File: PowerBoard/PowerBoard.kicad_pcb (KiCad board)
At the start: 2 copper layers, 45 x 100 mm, 13 parts, among them U1 RDE20110S12

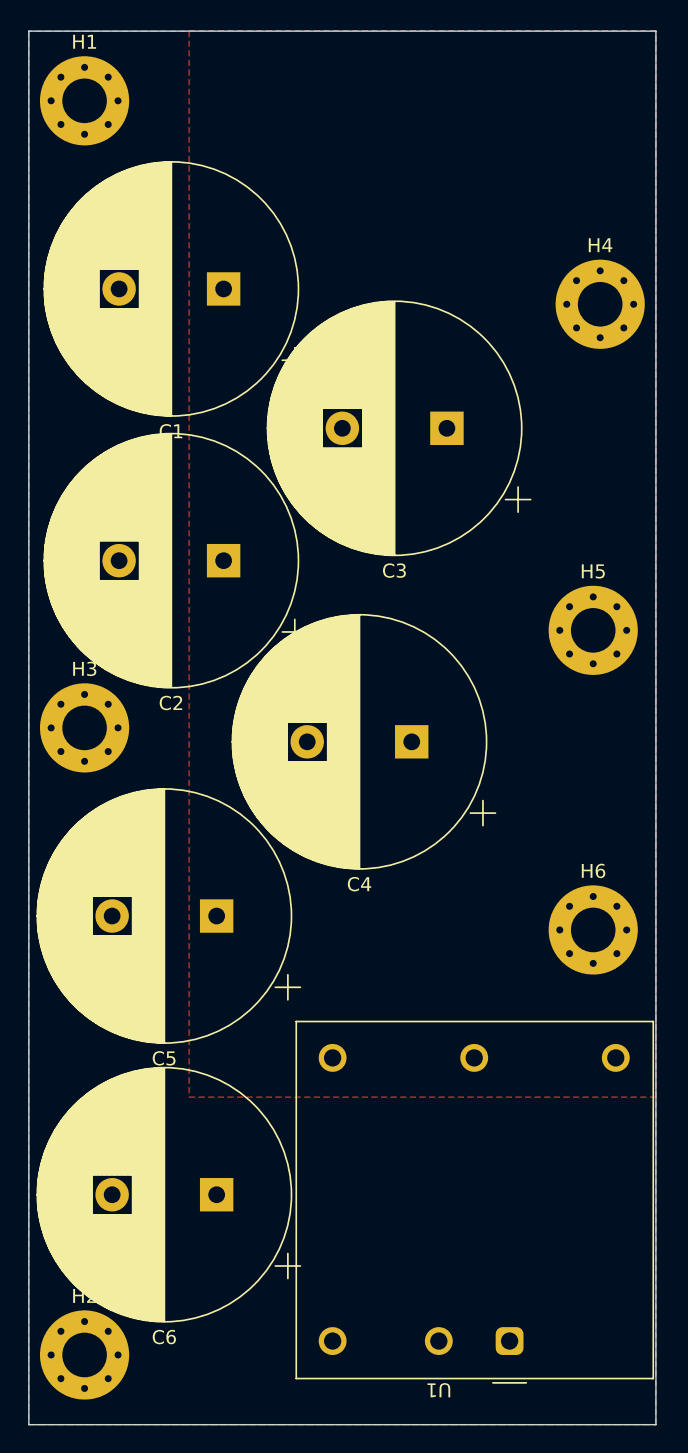
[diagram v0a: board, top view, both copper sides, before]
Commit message: cheap_board
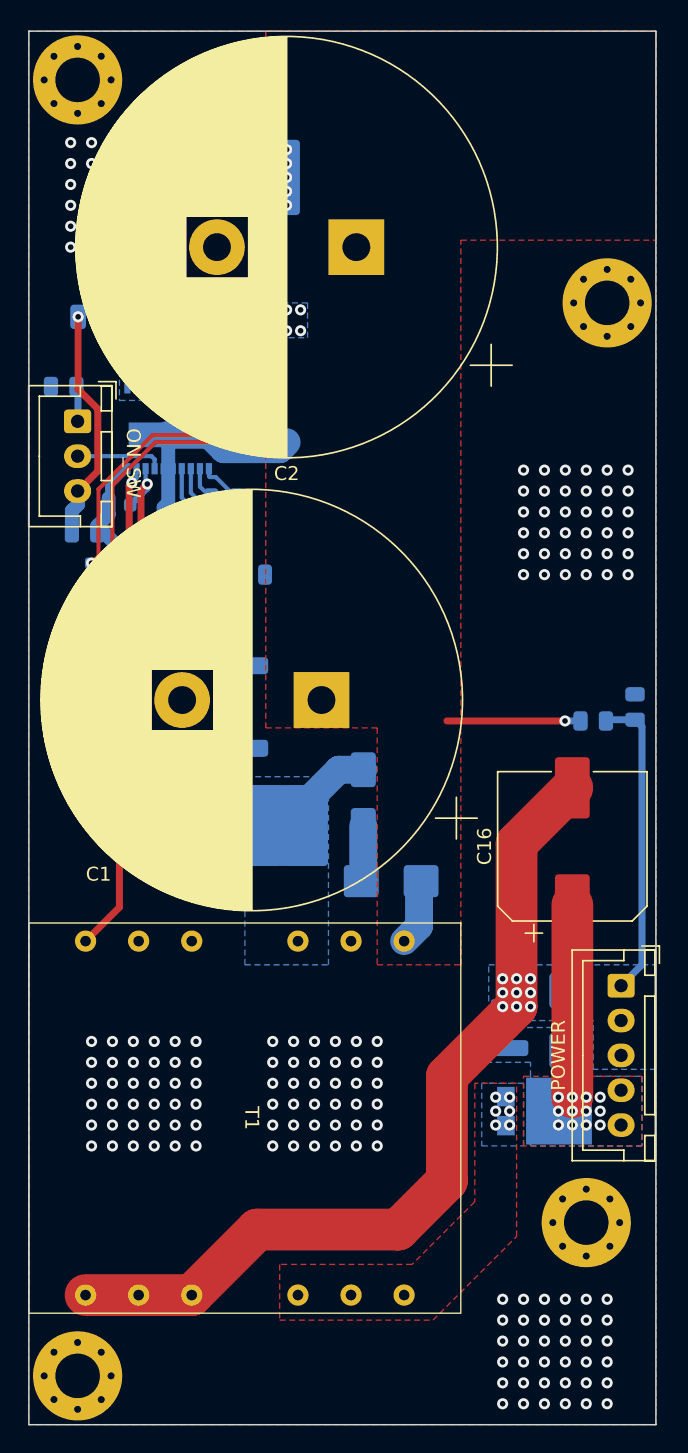
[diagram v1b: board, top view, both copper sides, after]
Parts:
- removed C3, C4, C5, C6: 680uF 200V, Capacitor_THT:CP_Radial_D18.0mm_P7.50mm
- removed H5, H6: BATT+Hole, MountingHole:MountingHole_3.2mm_M3_Pad_Via
- removed U1: RDE20110S12, Converter_DCDC:Converter_DCDC_TRACO_THN30-xxxx_THT
- added C10: 47p 25V, Capacitor_SMD:C_0805_2012Metric, B.Cu at (60.5, 87.0)
- added C11: 4.7u 50V, Capacitor_SMD:C_1206_3216Metric, B.Cu at (66.0, 77.5)
- added C12: 47p 100V, Capacitor_SMD:C_0603_1608Metric, B.Cu at (56.5, 93.0)
- added C13: 1n, Capacitor_SMD:C_0603_1608Metric, B.Cu at (56.5, 84.0)
- added C14: 2.2nF, Capacitor_SMD:C_0805_2012Metric, B.Cu at (85.0, 116.5)
- added C15: 47u 16V, Capacitor_SMD:C_1210_3225Metric, B.Cu at (84.5, 121.5)
- added C16: 470u 25V, Capacitor_SMD:CP_Elec_10x10.5, F.Cu at (89.0, 108.5)
- added C17: 4.7u 50V, Capacitor_SMD:C_1206_3216Metric, B.Cu at (66.0, 75.0)
- added C7: 1u 200V, Capacitor_SMD:C_2220_5650Metric, B.Cu at (66.0, 60.5)
- added C8: 100n 200V, Capacitor_SMD:C_0805_2012Metric, B.Cu at (59.0, 68.5)
- added C9: 100n, Capacitor_SMD:C_0805_2012Metric, B.Cu at (66.0, 89.0)
- added D1: BAV20WS-7-F, Diode_SMD:D_SOD-323, B.Cu at (54.5, 92.5)
- added D2: US1M, Diode_SMD:D_SMA, B.Cu at (74.0, 105.0)
- added D3: SMBJ188A, Diode_SMD:D_SMB, B.Cu at (76.0, 111.0)
- added D4: FSV15120V, Package_TO_SOT_SMD:TO-277A, B.Cu at (87.0, 127.5)
- added D5: 3SMB5928B, Diode_SMD:D_SMB, B.Cu at (88.5, 121.0)
- added J1: AuxConn, Connector_JST:JST_XH_B5B-XH-A_1x05_P2.50mm_Vertical, F.Cu at (92.5, 118.5)
- added Q1: STD11N65M2, Package_TO_SOT_SMD:TO-252-3_TabPin2, B.Cu at (67.0, 107.0)
- added R1: 100k, Resistor_SMD:R_0805_2012Metric, B.Cu at (90.5, 99.5)
- added R10: 121k, Resistor_SMD:R_0805_2012Metric, B.Cu at (64.0, 83.5)
- added R11: 4.99k, Resistor_SMD:R_0805_2012Metric, B.Cu at (64.0, 85.5)
- added R12: 44.2k, Resistor_SMD:R_0805_2012Metric, B.Cu at (58.5, 90.0)
- added R13: 20, Resistor_SMD:R_0805_2012Metric, B.Cu at (59.5, 108.5)
- added R14: 100, Resistor_SMD:R_0805_2012Metric, B.Cu at (59.5, 103.5)
- added R15: 0.05, Resistor_SMD:R_2512_6332Metric, B.Cu at (65.5, 98.5)
- added R16: 20k, Resistor_SMD:R_0805_2012Metric, B.Cu at (54.0, 86.0)
- added R2: 1.8k, Resistor_SMD:R_0805_2012Metric, B.Cu at (93.5, 98.5)
- added R3: 499k, Resistor_SMD:R_1206_3216Metric, B.Cu at (55.0, 70.5)
- added R4: 20k, Resistor_SMD:R_0805_2012Metric, B.Cu at (52.5, 75.5)
- added R6: 10k, Resistor_SMD:R_0805_2012Metric, B.Cu at (62.5, 89.0)
- added R7: 56.2k, Resistor_SMD:R_0603_1608Metric, B.Cu at (60.5, 85.0)
- added R8: 10, Resistor_SMD:R_0603_1608Metric, B.Cu at (54.5, 89.0)
- added R9: 10k, Resistor_SMD:R_0603_1608Metric, B.Cu at (56.5, 90.0)
- added SW1: POWER_SW, Connector_JST:JST_XH_B3B-XH-A_1x03_P2.50mm_Vertical, F.Cu at (53.5, 78.0)
- added T1: 11328-T078, GigaVescLibs:PQ2620, F.Cu at (65.5, 128.0)
- added U2: LT8316EFE#PBF, GigaVescLibs:IC_LT8316EFE#PBF, B.Cu at (60.0, 78.5)
- C1, C2: footprint Capacitor_THT:CP_Radial_D18.0mm_P7.50mm -> Capacitor_THT:CP_Radial_D30.0mm_P10.00mm_SnapIn
- H4: value BATT+Hole -> BATT-Hole
- moved H4 85.6 mm to (53.5, 146.5)
- moved H3 48.3 mm to (91.5, 69.5)
- moved H2 37.2 mm to (90.0, 135.5)
- moved C1 30.3 mm to (71.0, 98.0)
- moved C2 24.4 mm to (73.5, 65.5)
- moved H1 1.58 mm to (53.5, 53.5)
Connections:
- H3 pad 1: -BATT -> unconnected-(H3-Pad1)
- H4 pad 1: +BATT -> -BATT
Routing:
- net GND: track 0.00 -> 61.3 mm, vias 0 -> 9
- net Net-(D1-A): track 0.00 -> 29.8 mm, vias 0 -> 1
- net -BATT: track 0.00 -> 28.1 mm, vias 0 -> 180
- net Net-(U2-GATE): track 0.00 -> 27.4 mm, vias 0 -> 2
- net Net-(U2-SENSE): track 0.00 -> 24.0 mm, vias 0 -> 2
- net IN_V: track 0.00 -> 22.0 mm
- net Net-(U2-DCM): track 0.00 -> 21.9 mm, vias 0 -> 2
- net Net-(U2-BIAS): track 0.00 -> 20.8 mm, vias 0 -> 2
- net Net-(SW1-C): track 0.00 -> 16.4 mm, vias 0 -> 1
- net +BATT: track 0.00 -> 14.4 mm, vias 0 -> 12
- net +12V: track 0.00 -> 13.8 mm, vias 0 -> 12
- net Net-(U2-FB): track 0.00 -> 13.4 mm
- net Net-(D2-A): track 0.00 -> 11.6 mm
- net Net-(U2-VC): track 0.00 -> 8.10 mm
- net Net-(Q1-S): track 0.00 -> 7.85 mm
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- added copper zone on B.Cu, net +12V
- added copper zone on F.Cu, net +12V
- added copper zone on B.Cu, net +BATT
- added copper zone on F.Cu, net -BATT
- added copper zone on B.Cu, net GND
- added copper zone on B.Cu, net Net-(D2-A)
- added copper zone on B.Cu, net Net-(D4-A-Pad1)
- added copper zone on F.Cu, net Net-(D4-A-Pad1)
